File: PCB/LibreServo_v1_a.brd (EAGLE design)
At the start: 44.5 x 61.5 mm, 78 parts

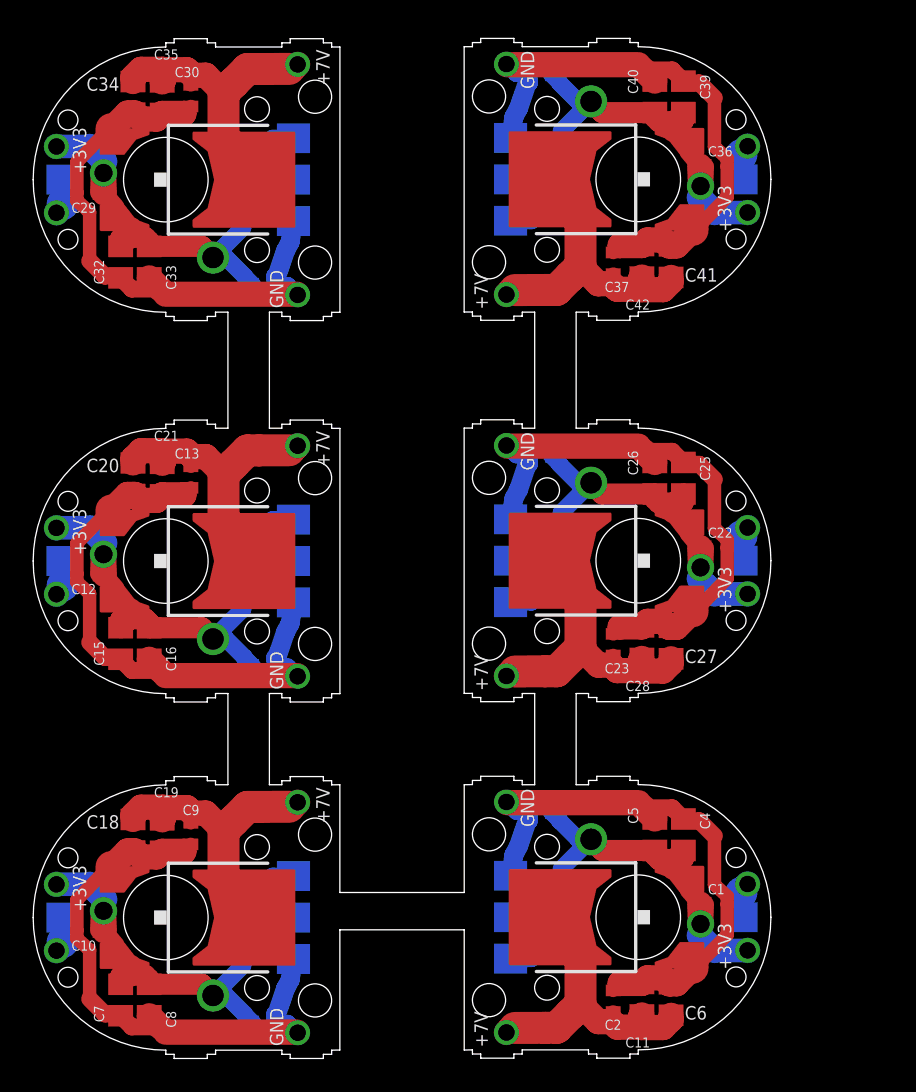
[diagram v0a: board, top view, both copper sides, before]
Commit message: LibreServo v1.c
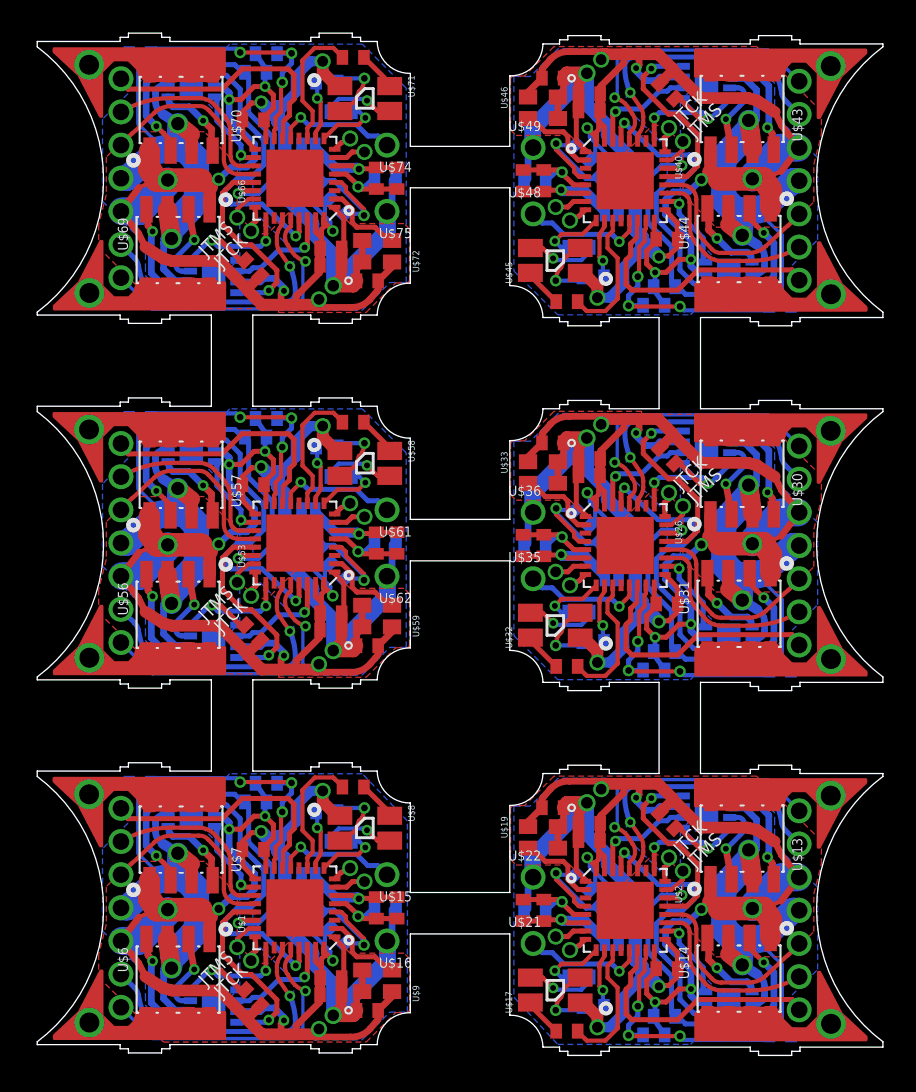
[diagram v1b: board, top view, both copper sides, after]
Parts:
- added R1, R10, R11, R12, R13, R15, R16, R17, R19, R20, R21, R23, R24, R3, R4, R5, R7, R9: 10K, rcl:R0402
- added R14, R18, R2, R22, R6, R8: 51K, rcl:R0402
- added R_BLUE, R_BLUE1, R_BLUE2, R_BLUE3, R_BLUE4, R_BLUE5: 470, rcl:R0402
- added R_GREEN, R_GREEN1, R_GREEN2, R_GREEN3, R_GREEN4, R_GREEN5: 300, rcl:R0402
- added R_RED, R_RED1, R_RED2, R_RED3, R_RED4, R_RED5: 330, rcl:R0402
- added SJ1, SJ11, SJ3, SJ5, SJ7, SJ9: SOLDAR, SparkFun-Passives:SJ_2S
- added SJ10, SJ12, SJ2, SJ4, SJ6, SJ8: NO-SOLDAR, SparkFun-Passives:SJ_2S-NO
- added U$37, U$50, U$63, U$76: HEADER_7_MIN, Propio:HEADER_7_MIN
- added U$38, U$51, U$64, U$77: PAD_LIBRE_SERVO_V1_A, Propio:PAD_LIBRE_SERVO_V1_A
- added U$39, U$52, U$65, U$78: PAD_LIBRE_SERVO_V1_B, Propio:PAD_LIBRE_SERVO_V1_B
- added U$40, U$53, U$66: STM32F302, Propio:QFN32
- added U$41, U$42, U$54, U$55, U$67, U$68: FAN3227/3, Propio:MLP8
- added U$43, U$44, U$56, U$57, U$69, U$70: FDS8858CZ, Propio:SO-8
- added U$45, U$58, U$71: RGB_PLCC4, Propio:PLCC4
- added U$46, U$59, U$72: OSC-8MHz, Propio:OSC-2.5X2
- added U$47, U$60, U$73: FERRITA, Propio:0402
- added U$48, U$49, U$61, U$62, U$74, U$75: HEADER_1_MIN, Propio:HEADER_1_MIN
- C10: value 100nF -> 1uF
- C11, C16, C19, C20, C21, C26, C27, C28, C33, C34, C35, C4, C40, C41, C42, C6, C7: value 10uF -> 100nF; device rcl:C0805 -> rcl:C0402
- C15, C8: value 10uF -> 4.7uF; device rcl:C0805 -> rcl:C0402
- C18, C25, C32, C39, C5: value 10uF -> 1uF; device rcl:C0805 -> rcl:C0402
- C23, C3, C30, C37: value 100nF -> 4.7uF
- U$1: value MURATA_SV01 -> STM32F302; device Propio:MURATA_SV01 -> Propio:QFN32
- U$10, U$11, U$12, U$29: value HEADER_1_MIN -> FAN3227/3; device Propio:HEADER_1_MIN -> Propio:MLP8
- U$13, U$30, U$7: value NCP1117DT33G -> FDS8858CZ; device Propio:DPAK_SP -> Propio:SO-8
- U$14, U$31: value MURATA_SV01 -> FDS8858CZ; device Propio:MURATA_SV01 -> Propio:SO-8
- U$17, U$32: value HEADER_1_MIN -> RGB_PLCC4; device Propio:HEADER_1_MIN -> Propio:PLCC4
- U$18, U$23: value HEADER_1_MIN -> HEADER_7_MIN; device Propio:HEADER_1_MIN -> Propio:HEADER_7_MIN
- U$19: value NCP1117DT33G -> OSC-8MHz; device Propio:DPAK_SP -> Propio:OSC-2.5X2
- U$2, U$26: value HEADER_1_MIN -> STM32F302; device Propio:HEADER_1_MIN -> Propio:QFN32
- U$20: value MURATA_SV01 -> FERRITA; device Propio:MURATA_SV01 -> Propio:0402
- U$24, U$4: value HEADER_1_MIN -> PAD_LIBRE_SERVO_V1_A; device Propio:HEADER_1_MIN -> Propio:PAD_LIBRE_SERVO_V1_A
- U$25, U$28: value HEADER_1_MIN -> PAD_LIBRE_SERVO_V1_B; device Propio:HEADER_1_MIN -> Propio:PAD_LIBRE_SERVO_V1_B
- U$27: value NCP1117DT33G -> FAN3227/3; device Propio:DPAK_SP -> Propio:MLP8
- U$3: value MURATA_SV01 -> FAN3227/3; device Propio:MURATA_SV01 -> Propio:MLP8
- U$33, U$9: value HEADER_1_MIN -> OSC-8MHz; device Propio:HEADER_1_MIN -> Propio:OSC-2.5X2
- U$34, U$5: value HEADER_1_MIN -> FERRITA; device Propio:HEADER_1_MIN -> Propio:0402
- U$36: value NCP1117DT33G -> HEADER_1_MIN; device Propio:DPAK_SP -> Propio:HEADER_1_MIN
- U$6: value HEADER_1_MIN -> FDS8858CZ; device Propio:HEADER_1_MIN -> Propio:SO-8
- U$8: value MURATA_SV01 -> RGB_PLCC4; device Propio:MURATA_SV01 -> Propio:PLCC4
- moved U$24 63.7 mm to (42.2, 1.80)
- moved U$21 56.0 mm to (30.4, 6.92)
- moved U$20 49.4 mm to (30.5, 8.89), turned to 180 degrees
- moved U$10 47.6 mm to (42.2, 3.04), flipped to the bottom, turned to 180 degrees
- moved U$23 45.6 mm to (46.5, 14.9), turned to 270 degrees
- moved U$28 44.6 mm to (9.82, 1.88), turned to 180 degrees
- moved U$29 43.5 mm to (42.2, 25.0), flipped to the bottom, turned to 180 degrees
- moved C12 42.3 mm to (38.5, 5.40), turned to 0 degrees
- moved U$27 41.5 mm to (40.9, 36.9), flipped to the bottom, turned to 180 degrees
- moved U$30 37.0 mm to (43.0, 35.3), turned to 90 degrees
- moved U$13 36.5 mm to (43.0, 13.3), turned to 90 degrees
- moved U$4 34.0 mm to (9.80, 16.2)
- moved C13 34.0 mm to (33.4, 10.6), flipped to the bottom, turned to 225 degrees
- moved U$9 33.5 mm to (21.0, 4.67), turned to 90 degrees
- moved C19 33.4 mm to (31.6, 37.1), turned to 180 degrees
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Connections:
- removed net GND1: C1.2, C11.1, C2.1, C3.2, C4.2, C5.2, C6.1, U$1.P$3, U$5.P$1, U$7.1
- removed net GND2: C12.2, C13.1, C14.2, C15.2, C16.2, C20.1, C21.1, U$11.P$1, U$13.1, U$8.P$3
- removed net GND3: C10.2, C17.2, C18.1, C19.1, C7.2, C8.2, C9.1, U$25.P$1, U$27.1, U$3.P$3
- removed net GND4: C22.2, C23.1, C24.2, C25.2, C26.2, C27.1, C28.1, U$14.P$3, U$17.P$1, U$19.1
- removed net GND5: C29.2, C30.1, C31.2, C32.2, C33.2, C34.1, C35.1, U$20.P$3, U$28.P$1, U$30.1
- removed net GND6: C36.2, C37.1, C38.2, C39.2, C40.2, C41.1, C42.1, U$31.P$3, U$34.P$1, U$36.1
- new net EN_Q1: R9.2, U$1.25, U$11.P$1, U$11.P$8
- new net EN_Q10: R20.1, U$53.22, U$55.P$1, U$55.P$8
- new net EN_Q11: R23.2, U$66.25, U$67.P$1, U$67.P$8
- new net EN_Q12: R24.1, U$66.22, U$68.P$1, U$68.P$8
- new net EN_Q2: R10.1, U$1.22, U$12.P$1, U$12.P$8
- new net EN_Q3: R3.2, U$2.25, U$3.P$1, U$3.P$8
- new net EN_Q4: R4.1, U$10.P$1, U$10.P$8, U$2.22
- new net EN_Q5: R11.2, U$26.25, U$27.P$1, U$27.P$8
- new net EN_Q6: R12.1, U$26.22, U$29.P$1, U$29.P$8
- new net EN_Q7: R15.2, U$40.25, U$41.P$1, U$41.P$8
- new net EN_Q8: R16.1, U$40.22, U$42.P$1, U$42.P$8
- new net EN_Q9: R19.2, U$53.25, U$54.P$1, U$54.P$8
- new net EN_SERIAL_1: U$1.28, U$18.P$1
- new net EN_SERIAL_2: U$2.28, U$23.P$1
- new net EN_SERIAL_3: U$26.28, U$37.P$1
- new net EN_SERIAL_4: U$40.28, U$50.P$1
- new net EN_SERIAL_5: U$53.28, U$63.P$1
- new net EN_SERIAL_6: U$66.28, U$76.P$1
- new net GNDA: C4.2, C5.2, SJ1.2, U$1.6
- new net GNDA1: C10.2, C9.2, SJ3.2, U$2.6
- new net GNDA2: C17.2, C18.2, SJ5.2, U$26.6
- new net GNDA3: C24.2, C25.2, SJ7.2, U$40.6
- new net GNDA4: C31.2, C32.2, SJ9.2, U$53.6
- new net GNDA5: C38.2, C39.2, SJ11.2, U$66.6
- new net GND_1: C1.1, C16.2, C2.2, C3.1, C6.2, R10.2, R7.2, R9.1, SJ1.1, SJ2.1, U$1.16, U$1.31, U$1.32, U$11.P$3, U$12.P$3, U$18.P$3, U$6.P$1, U$7.P$1, U$9.P$2
- new net GND_2: C11.2, C12.1, C13.2, C7.2, C8.1, R1.2, R3.1, R4.2, SJ3.1, SJ4.1, U$10.P$3, U$13.P$1, U$14.P$1, U$19.P$2, U$2.16, U$2.31, U$2.32, U$23.P$3, U$3.P$3
- new net GND_3: C14.2, C15.1, C19.2, C20.1, C21.2, R11.1, R12.2, R5.2, SJ5.1, SJ6.1, U$26.16, U$26.31, U$26.32, U$27.P$3, U$29.P$3, U$30.P$1, U$31.P$1, U$33.P$2, U$37.P$3
- new net GND_4: C22.2, C23.1, C26.2, C27.1, C28.2, R13.2, R15.1, R16.2, SJ7.1, SJ8.1, U$40.16, U$40.31, U$40.32, U$41.P$3, U$42.P$3, U$43.P$1, U$44.P$1, U$46.P$2, U$50.P$3
- new net GND_5: C29.2, C30.1, C33.2, C34.1, C35.2, R17.2, R19.1, R20.2, SJ10.1, SJ9.1, U$53.16, U$53.31, U$53.32, U$54.P$3, U$55.P$3, U$56.P$1, U$57.P$1, U$59.P$2, U$63.P$3
- new net GND_6: C36.2, C37.1, C40.2, C41.1, C42.2, R21.2, R23.1, R24.2, SJ11.1, SJ12.1, U$66.16, U$66.31, U$66.32, U$67.P$3, U$68.P$3, U$69.P$1, U$70.P$1, U$72.P$2, U$76.P$3
- new net JTCK: U$1.24
- new net JTCK1: U$2.24
- new net JTCK2: U$26.24
- new net JTCK3: U$40.24
- new net JTCK4: U$53.24
- new net JTCK5: U$66.24
- new net JTMS: U$1.23
- new net JTMS1: U$2.23
- new net JTMS2: U$26.23
- new net JTMS3: U$40.23
- new net JTMS4: U$53.23
- new net JTMS5: U$66.23
- new net LED_BLUE: R_BLUE.2, U$1.11
- new net LED_BLUE1: R_BLUE1.2, U$2.11
- new net LED_BLUE2: R_BLUE2.2, U$26.11
- new net LED_BLUE3: R_BLUE3.2, U$40.11
- new net LED_BLUE4: R_BLUE4.2, U$53.11
- new net LED_BLUE5: R_BLUE5.2, U$66.11
- new net LED_GREEN: R_GREEN.2, U$1.9
- new net LED_GREEN1: R_GREEN1.2, U$2.9
- new net LED_GREEN2: R_GREEN2.2, U$26.9
- new net LED_GREEN3: R_GREEN3.2, U$40.9
- new net LED_GREEN4: R_GREEN4.2, U$53.9
- new net LED_GREEN5: R_GREEN5.2, U$66.9
- new net LED_RED: R_RED.2, U$1.10
- new net LED_RED1: R_RED1.2, U$2.10
- new net LED_RED2: R_RED2.2, U$26.10
- new net LED_RED3: R_RED3.2, U$40.10
- new net LED_RED4: R_RED4.2, U$53.10
- new net LED_RED5: R_RED5.2, U$66.10
- new net N$1: R_BLUE.1, U$8.P$2
- new net N$10: U$11.P$7, U$6.P$2
- new net N$11: U$10.P$7, U$14.P$2
- new net N$12: U$10.P$5, U$14.P$4
- new net N$13: U$13.P$5, U$13.P$6, U$13.P$7, U$13.P$8, U$25.P$1, U$25.P$2
- new net N$14: U$11.P$5, U$6.P$4
- new net N$15: U$12.P$7, U$7.P$2
- new net N$16: U$14.P$5, U$14.P$6, U$14.P$7, U$14.P$8, U$24.P$1, U$24.P$2
- new net N$17: R_BLUE1.1, U$17.P$2
- new net N$18: U$12.P$5, U$7.P$4
- new net N$19: U$28.P$1, U$28.P$2, U$6.P$5, U$6.P$6, U$6.P$7, U$6.P$8
- new net N$2: R_GREEN.1, U$8.P$3
- new net N$20: R_GREEN1.1, U$17.P$3
- new net N$21: R_RED1.1, U$17.P$4
- new net N$22: U$2.8
- new net N$23: U$2.7
- new net N$24: U$26.2, U$33.P$3
- new net N$25: U$27.P$7, U$30.P$2
- new net N$26: U$4.P$1, U$4.P$2, U$7.P$5, U$7.P$6, U$7.P$7, U$7.P$8
- new net N$27: U$27.P$5, U$30.P$4
- new net N$28: U$29.P$7, U$31.P$2
- new net N$29: U$29.P$5, U$31.P$4
- new net N$3: R_RED.1, U$8.P$4
- new net N$30: U$30.P$5, U$30.P$6, U$30.P$7, U$30.P$8, U$39.P$1, U$39.P$2
- new net N$31: U$31.P$5, U$31.P$6, U$31.P$7, U$31.P$8, U$38.P$1, U$38.P$2
- new net N$32: R_BLUE2.1, U$32.P$2
- new net N$33: R_GREEN2.1, U$32.P$3
- new net N$34: R_RED2.1, U$32.P$4
- new net N$35: U$26.8
- new net N$36: U$26.7
- new net N$37: U$40.2, U$46.P$3
- new net N$38: U$41.P$7, U$43.P$2
- new net N$39: U$41.P$5, U$43.P$4
- new net N$4: U$19.P$3, U$2.2
- new net N$40: U$42.P$7, U$44.P$2
- new net N$41: U$42.P$5, U$44.P$4
- new net N$42: U$43.P$5, U$43.P$6, U$43.P$7, U$43.P$8, U$52.P$1, U$52.P$2
- new net N$43: U$44.P$5, U$44.P$6, U$44.P$7, U$44.P$8, U$51.P$1, U$51.P$2
- new net N$44: R_BLUE3.1, U$45.P$2
- new net N$45: R_GREEN3.1, U$45.P$3
- new net N$46: R_RED3.1, U$45.P$4
- new net N$47: U$40.8
- new net N$48: U$40.7
- new net N$49: U$53.2, U$59.P$3
- new net N$5: U$1.2, U$9.P$3
- new net N$50: U$54.P$7, U$56.P$2
- new net N$51: U$54.P$5, U$56.P$4
- new net N$52: U$55.P$7, U$57.P$2
- new net N$53: U$55.P$5, U$57.P$4
- new net N$54: U$56.P$5, U$56.P$6, U$56.P$7, U$56.P$8, U$65.P$1, U$65.P$2
- new net N$55: U$57.P$5, U$57.P$6, U$57.P$7, U$57.P$8, U$64.P$1, U$64.P$2
- new net N$56: R_BLUE4.1, U$58.P$2
- new net N$57: R_GREEN4.1, U$58.P$3
- new net N$58: R_RED4.1, U$58.P$4
- new net N$59: U$53.8
- new net N$6: U$1.8
- new net N$60: U$53.7
- new net N$61: U$66.2, U$72.P$3
- new net N$62: U$67.P$7, U$69.P$2
- new net N$63: U$67.P$5, U$69.P$4
- new net N$64: U$68.P$7, U$70.P$2
- new net N$65: U$68.P$5, U$70.P$4
- new net N$66: U$69.P$5, U$69.P$6, U$69.P$7, U$69.P$8, U$78.P$1, U$78.P$2
- new net N$67: U$70.P$5, U$70.P$6, U$70.P$7, U$70.P$8, U$77.P$1, U$77.P$2
- new net N$68: R_BLUE5.1, U$71.P$2
- new net N$69: R_GREEN5.1, U$71.P$3
- new net N$7: U$1.7
- new net N$70: R_RED5.1, U$71.P$4
- new net N$71: U$66.8
- new net N$72: U$66.7
- new net N$8: U$13.P$2, U$3.P$7
- new net N$9: U$13.P$4, U$3.P$5
- new net NRST: C16.1, SJ2.2, U$1.4
- new net NRST1: C13.1, SJ4.2, U$2.4
- new net NRST2: C21.1, SJ6.2, U$26.4
- new net NRST3: C28.1, SJ8.2, U$40.4
- new net NRST4: C35.1, SJ10.2, U$53.4
- new net NRST5: C42.1, SJ12.2, U$66.4
- new net Q1_INA_N: U$1.30, U$11.P$2
- new net Q1_INA_N1: U$2.30, U$3.P$2
- new net Q1_INA_N2: U$26.30, U$27.P$2
- new net Q1_INA_N3: U$40.30, U$41.P$2
- new net Q1_INA_N4: U$53.30, U$54.P$2
- new net Q1_INA_N5: U$66.30, U$67.P$2
- new net Q2_INA_N: U$1.29, U$12.P$2
- new net Q2_INA_N1: U$10.P$2, U$2.29
- new net Q2_INA_N2: U$26.29, U$29.P$2
- new net Q2_INA_N3: U$40.29, U$42.P$2
- new net Q2_INA_N4: U$53.29, U$55.P$2
- new net Q2_INA_N5: U$66.29, U$68.P$2
- new net RX_1: U$1.19, U$18.P$6
- new net RX_2: U$2.19, U$23.P$6
- new net RX_3: U$26.19, U$37.P$6
- new net RX_4: U$40.19, U$50.P$6
- new net RX_5: U$53.19, U$63.P$6
- new net RX_6: U$66.19, U$76.P$6
- new net TIM1_CH1: U$1.18, U$12.P$4
- new net TIM1_CH10: U$53.18, U$55.P$4
- new net TIM1_CH11: U$66.21, U$67.P$4
- new net TIM1_CH12: U$66.18, U$68.P$4
- new net TIM1_CH2: U$2.21, U$3.P$4
- new net TIM1_CH3: U$10.P$4, U$2.18
- new net TIM1_CH4: U$1.21, U$11.P$4
- new net TIM1_CH5: U$26.21, U$27.P$4
- new net TIM1_CH6: U$26.18, U$29.P$4
- new net TIM1_CH7: U$40.21, U$41.P$4
- new net TIM1_CH8: U$40.18, U$42.P$4
- new net TIM1_CH9: U$53.21, U$54.P$4
- new net TX_1: U$1.20, U$18.P$5
- new net TX_2: U$2.20, U$23.P$5
- new net TX_3: U$26.20, U$37.P$5
- new net TX_4: U$40.20, U$50.P$5
- new net TX_5: U$53.20, U$63.P$5
- new net TX_6: U$66.20, U$76.P$5
- new net USART2_RX_1: U$1.27, U$18.P$2
- new net USART2_RX_2: U$2.27, U$23.P$2
- new net USART2_RX_3: U$26.27, U$37.P$2
- new net USART2_RX_4: U$40.27, U$50.P$2
- new net USART2_RX_5: U$53.27, U$63.P$2
- new net USART2_RX_6: U$66.27, U$76.P$2
- new net VBAT: R7.1, R8.2, U$1.15
- new net VBAT1: R1.1, R2.2, U$2.15
- new net VBAT2: R5.1, R6.2, U$26.15
- new net VBAT3: R13.1, R14.2, U$40.15
- new net VBAT4: R17.1, R18.2, U$53.15
- new net VBAT5: R21.1, R22.2, U$66.15
- new net VDD: C4.1, C5.1, U$1.5, U$5.2
- new net VDD1: C10.1, C9.1, U$2.5, U$20.2
- new net VDD2: C17.1, C18.1, U$26.5, U$34.2
- new net VDD3: C24.1, C25.1, U$40.5, U$47.2
- new net VDD4: C31.1, C32.1, U$53.5, U$60.2
- new net VDD5: C38.1, C39.1, U$66.5, U$73.2
- new net V_CORRIENTE_1: U$1.14, U$18.P$7
- new net V_CORRIENTE_2: U$2.14, U$23.P$7
- new net V_CORRIENTE_3: U$26.14, U$37.P$7
- new net V_CORRIENTE_4: U$40.14, U$50.P$7
- new net V_CORRIENTE_5: U$53.14, U$63.P$7
- new net V_CORRIENTE_6: U$66.14, U$76.P$7
- net +3V3_1: now also C1.2, C2.1, C3.2, C6.1, U$1.1, U$1.17, U$16.P$1, U$5.1, U$8.P$1, U$9.P$1, U$9.P$4; no longer C1.1, C3.1, C4.1, C5.1, U$1.P$1, U$2.P$1, U$7.3
- net +3V3_2: now also C11.1, C12.2, C7.1, C8.2, U$17.P$1, U$19.P$1, U$19.P$4, U$2.1, U$2.17, U$20.1, U$22.P$1; no longer C12.1, C14.1, C15.1, C16.1, U$13.3, U$8.P$1, U$9.P$1
- net +3V3_3: now also C14.1, C15.2, C19.1, C20.2, U$26.1, U$26.17, U$32.P$1, U$33.P$1, U$33.P$4, U$34.1, U$36.P$1; no longer C10.1, C17.1, C7.1, C8.1, U$22.P$1, U$27.3, U$3.P$1
- net +3V3_4: now also C23.2, C27.2, U$40.1, U$40.17, U$45.P$1, U$46.P$1, U$46.P$4, U$47.1, U$49.P$1; no longer C24.1, C25.1, U$14.P$1, U$15.P$1, U$19.3
- net +3V3_5: now also C30.2, C34.2, U$53.1, U$53.17, U$58.P$1, U$59.P$1, U$59.P$4, U$60.1, U$62.P$1; no longer C31.1, C32.1, U$20.P$1, U$21.P$1, U$30.3
- net +3V3_6: now also C37.2, C41.2, U$66.1, U$66.17, U$71.P$1, U$72.P$1, U$72.P$4, U$73.1, U$75.P$1; no longer C38.1, C39.1, U$31.P$1, U$32.P$1, U$36.3
- net +7V_1: now also R8.1, U$11.P$6, U$12.P$6, U$18.P$4, U$6.P$3, U$7.P$3; no longer C11.2, C2.2, C6.2, U$6.P$1, U$7.4
- net +7V_2: now also R2.1, U$10.P$6, U$13.P$3, U$14.P$3, U$23.P$4, U$3.P$6; no longer C13.2, C20.2, C21.2, U$12.P$1, U$13.4
- net +7V_3: now also R6.1, U$27.P$6, U$29.P$6, U$30.P$3, U$31.P$3, U$37.P$4; no longer C18.2, C19.2, C9.2, U$26.P$1, U$27.4
- net +7V_4: now also R14.1, U$41.P$6, U$42.P$6, U$43.P$3, U$44.P$3, U$50.P$4; no longer C23.2, C27.2, C28.2, U$18.P$1, U$19.4
- net +7V_5: now also R18.1, U$54.P$6, U$55.P$6, U$56.P$3, U$57.P$3, U$63.P$4; no longer C30.2, C34.2, C35.2, U$29.P$1, U$30.4
- net +7V_6: now also R22.1, U$67.P$6, U$68.P$6, U$69.P$3, U$70.P$3, U$76.P$4; no longer C37.2, C41.2, C42.2, U$35.P$1, U$36.4
- net V_POT_1: now also U$1.13, U$15.P$1; no longer U$1.P$4, U$4.P$1
- net V_POT_2: now also U$2.13, U$21.P$1; no longer U$10.P$1, U$8.P$4
- net V_POT_3: now also U$26.13, U$35.P$1; no longer U$23.P$1, U$3.P$4
- net V_POT_4: now also U$40.13, U$48.P$1; no longer U$14.P$4, U$16.P$1
- net V_POT_5: now also U$53.13, U$61.P$1; no longer U$20.P$4, U$24.P$1
- net V_POT_6: now also U$66.13, U$74.P$1; no longer U$31.P$4, U$33.P$1
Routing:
- net GND_5: track 0.00 -> 72.9 mm, vias 0 -> 7
- net GND_1: track 0.00 -> 72.9 mm, vias 0 -> 7
- net GND_6: track 0.00 -> 72.9 mm, vias 0 -> 7
- net GND_4: track 0.00 -> 72.9 mm, vias 0 -> 7
- net GND_3: track 0.00 -> 72.9 mm, vias 0 -> 7
- net GND_2: track 0.00 -> 72.9 mm, vias 0 -> 7
- net GND4: track 36.2 -> 0.00 mm
- net GND6: track 36.2 -> 0.00 mm
- net GND1: track 36.2 -> 0.00 mm
- net GND5: track 36.2 -> 0.00 mm
- net GND3: track 36.2 -> 0.00 mm
- net GND2: track 36.2 -> 0.00 mm
- net EN_SERIAL_4: track 0.00 -> 17.6 mm, vias 0 -> 1
- net EN_SERIAL_3: track 0.00 -> 17.6 mm, vias 0 -> 1
- net EN_SERIAL_2: track 0.00 -> 17.6 mm, vias 0 -> 1
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- added copper zone on layer 16, net +3V3_1
- added copper zone on layer 16, net +3V3_2
- added copper zone on layer 16, net +3V3_3
- added copper zone on layer 16, net +3V3_4
- added copper zone on layer 16, net +3V3_5
- added copper zone on layer 16, net +3V3_6
- added copper zone on layer 16, net +7V_1
- added copper zone on layer 16, net +7V_2
- added copper zone on layer 16, net +7V_3
- added copper zone on layer 16, net +7V_4
- added copper zone on layer 16, net +7V_5
- added copper zone on layer 16, net +7V_6
- added copper zone on layer 1, net GND_1
- added copper zone on layer 1, net GND_2
- added copper zone on layer 1, net GND_3
- added copper zone on layer 1, net GND_4
- added copper zone on layer 1, net GND_5
- added copper zone on layer 1, net GND_6
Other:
- board size 44.5 x 61.5 mm -> 51 x 61.7 mm
- board text added: "2x"
- board text added: "3V3"
- board text added: "3v3"
- board text added: "8MHz"
- board text added: "C1"
- board text added: "C16"
- board text added: "EN-S"
- board text added: "I"
- board text added: "JTCK"
- board text added: "JTMS"
- board text added: "LibreServo v1.c"
- board text added: "R-B"
- board text added: "R-G"
- board text added: "R8"
- board text added: "R9"
- board text added: "RGB"
- board text added: "RX"
- board text added: "R_RED"
- board text added: "TX"
- board text added: "TX-2"
- board text removed: "+3V3"
